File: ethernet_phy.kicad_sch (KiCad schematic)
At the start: 24 parts, among them U1 RTL8201F

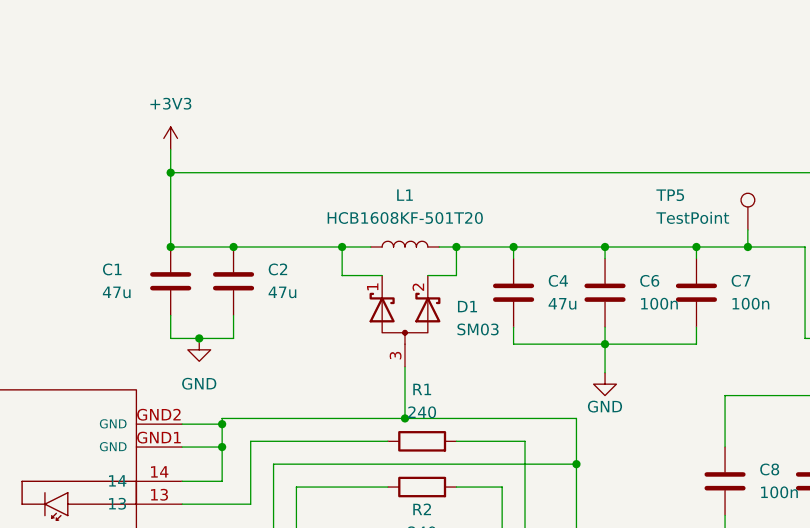
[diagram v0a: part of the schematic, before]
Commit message: Update kicad files
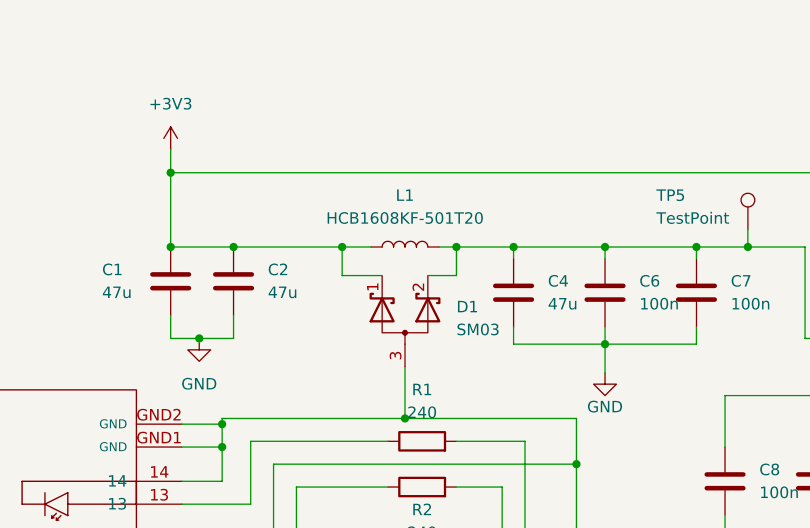
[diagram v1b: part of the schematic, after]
